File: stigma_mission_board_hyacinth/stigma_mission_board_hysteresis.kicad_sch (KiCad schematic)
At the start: 139 parts, among them J1 DF40C-70DS-0.4V(51), J10 JST-GH, J2 DF40C-70DS-0.4V(51), J6 SMA, J7 SMA, J8 RJ45_Wuerth_7499010211A, J9 JST-GH, Q1 AON7423, Q2 AO3400A, Q3 AO3401A, Q4 AO3400A, U10 MCP2562FD, U11 Ai-Thinker-Ra-01, U12 TPD4E1U06, U13 Ai-Thinker-Ra-01, U14 LAN8742A, U2 AZ1117I-3.3, U3 AZ1117I-3.3, U4 INA181A1, U6 AZ1117I-3.3, U7 AZ1117I-3.3, U8 MCP2562FD, U9 INA181A1, Y1 25MHz

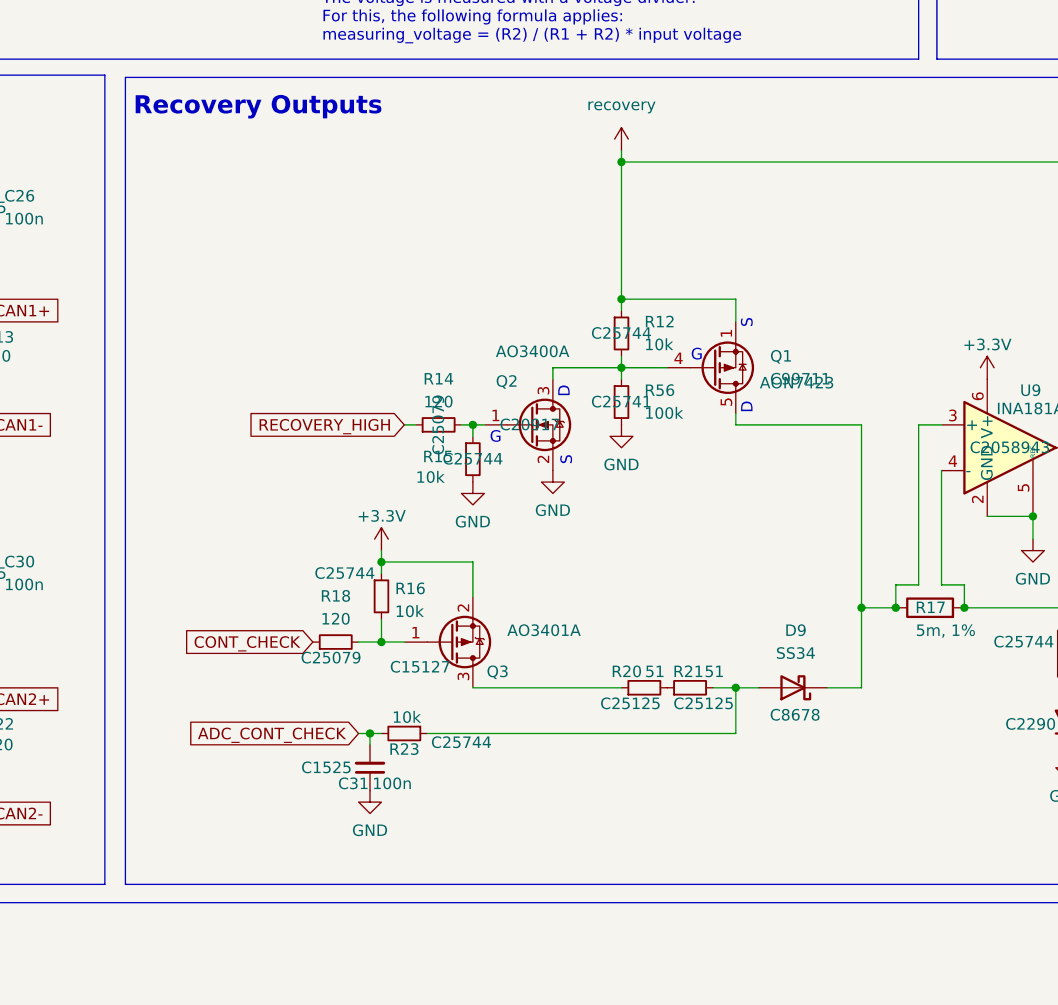
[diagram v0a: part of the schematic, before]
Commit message: remove cont check and rec jumper
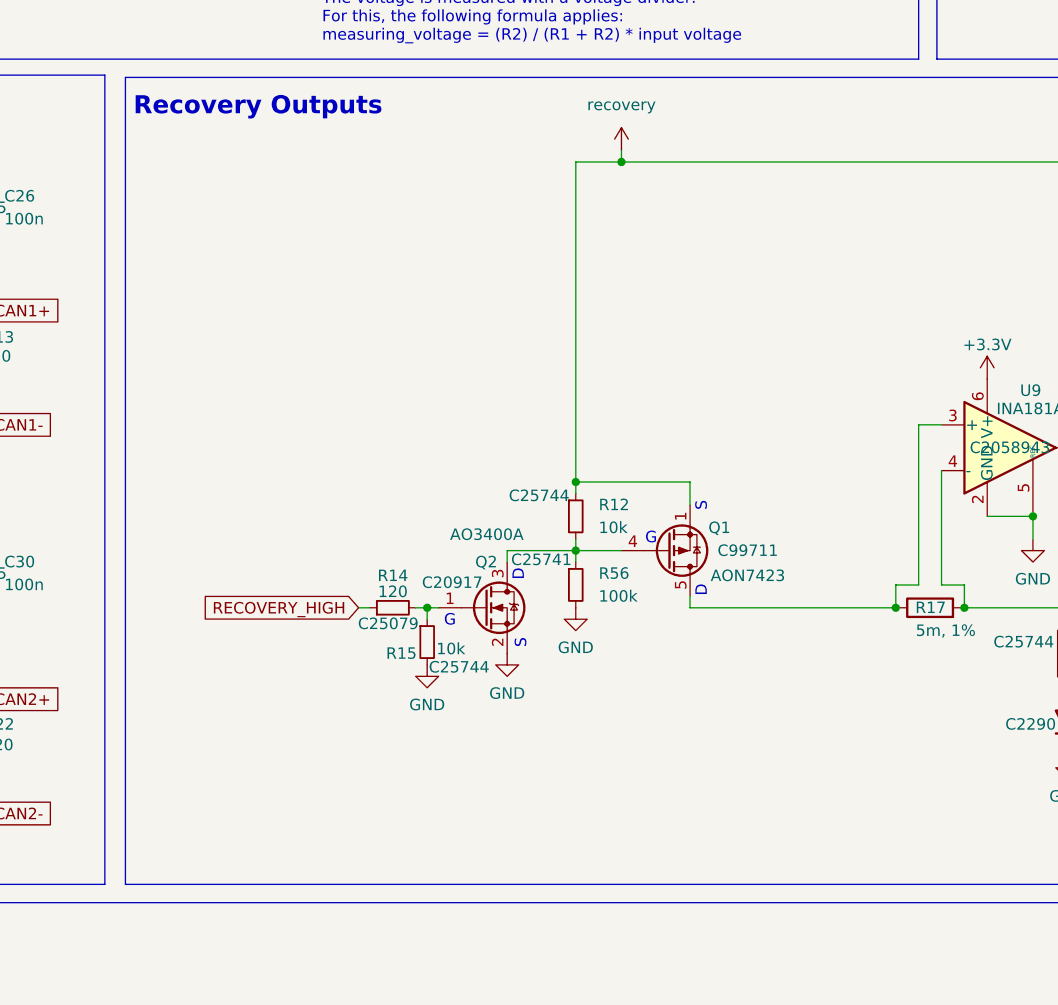
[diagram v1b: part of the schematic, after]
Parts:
- removed C31: 100n, Capacitor_SMD:C_0402_1005Metric, symbol Device:C_Small
- removed D9: SS34, Diode_SMD:D_SMA, symbol Diode:SS34
- removed Q3: AO3401A, Package_TO_SOT_SMD:SOT-23, symbol Transistor_FET:AO3401A
- removed R16, R23: 10k, Resistor_SMD:R_0402_1005Metric, symbol Device:R_Small
- removed R18: 120, Resistor_SMD:R_0402_1005Metric, symbol Device:R_Small
- removed R20, R21: 51, Resistor_SMD:R_0402_1005Metric, symbol Device:R_Small
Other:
- moved on the sheet: Q1, Q2, R12, R14, R15, R56
